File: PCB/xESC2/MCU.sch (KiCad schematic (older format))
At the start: 1 part, among them U4 STM32F405RGTx

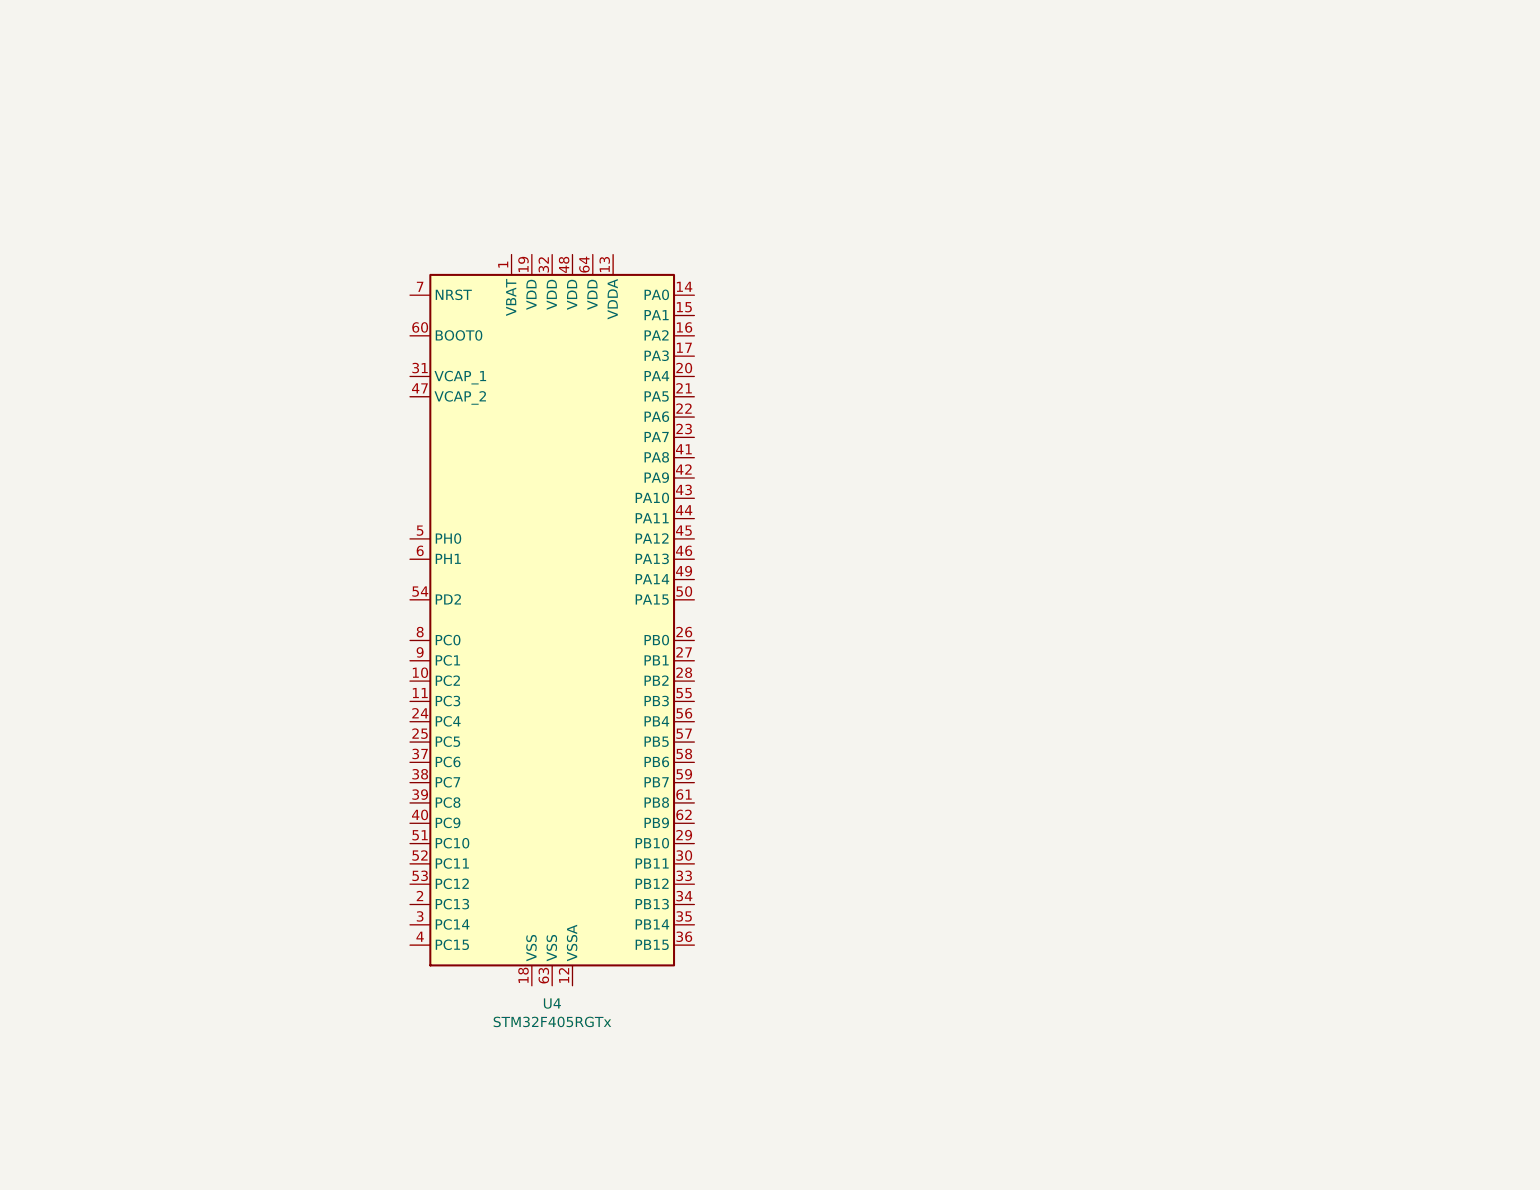
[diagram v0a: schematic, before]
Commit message: wip xESC2 logic
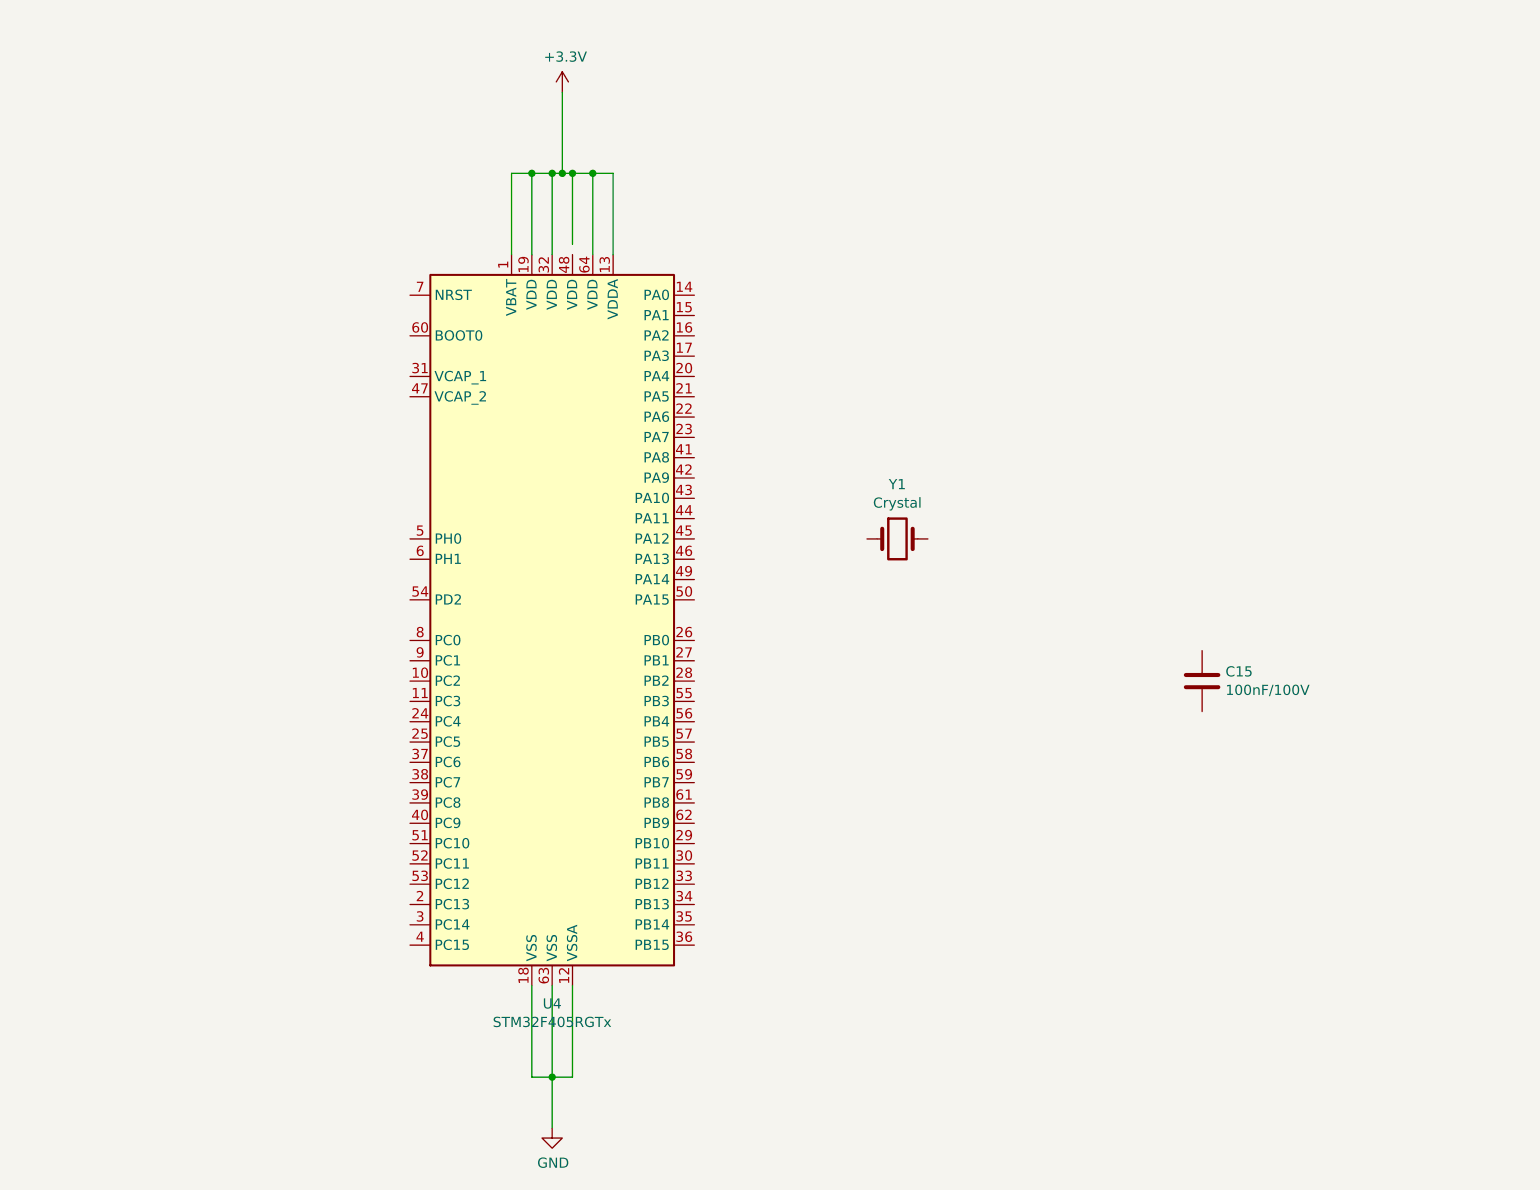
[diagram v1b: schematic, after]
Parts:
- added C15: 100nF/100V, Capacitor_SMD:C_0805_2012Metric, symbol Device:C
- added Y1: Crystal, Crystal:Crystal_SMD_HC49-SD, symbol Device:Crystal
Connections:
- net labels added: +3.3V, GND
- wire segments 0 -> 19
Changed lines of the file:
@@
+	1    0    0    -1
+$EndComp
+Wire Wire Line
+	3250 5150 3250 5600
+Wire Wire Line
+	3250 5600 3350 5600
+Wire Wire Line
+	3450 5600 3450 5150
+Wire Wire Line
+	3350 5150 3350 5600
+Connection ~ 3350 5600
+Wire Wire Line
+	3350 5600 3450 5600
+Wire Wire Line
+	3350 5600 3350 5850
+$Comp
+L power:GND #PWR0123
+U 1 1 61A9A167
+P 3350 5850
+F 0 "#PWR0123" H 3350 5600 50  0001 C CNN
+F 1 "GND" H 3355 5677 50  0000 C CNN
+F 2 "" H 3350 5850 50  0001 C CNN
+F 3 "" H 3350 5850 50  0001 C CNN
+	1    3350 5850
+	1    0    0    -1
+$EndComp
+$Comp
+L Device:C C?
+U 1 1 61A9BC8B
+P 6550 3650
+AR Path="/61A3F4E8/61A9BC8B" Ref="C?"  Part="1"
+AR Path="/61AC26FB/61A9BC8B" Ref="C15"  Part="1"
+F 0 "C15" H 6665 3696 50  0000 L CNN
+F 1 "100nF/100V" H 6665 3605 50  0000 L CNN
+F 2 "Capacitor_SMD:C_0805_2012Metric" H 6588 3500 50  0001 C CNN
+F 3 "~" H 6550 3650 50  0001 C CNN
+	1    6550 3650
+	1    0    0    -1
+$EndComp
+$Comp
+L power:+3.3V #PWR?
+U 1 1 61A9F4B2
+P 3400 750
+AR Path="/61A9F4B2" Ref="#PWR?"  Part="1"
+AR Path="/61AC26FB/61A9F4B2" Ref="#PWR0124"  Part="1"
+F 0 "#PWR0124" H 3400 600 50  0001 C CNN
+F 1 "+3.3V" H 3415 923 50  0000 C CNN
+F 2 "" H 3400 750 50  0001 C CNN
+F 3 "" H 3400 750 50  0001 C CNN
+	1    3400 750
+	1    0    0    -1
+$EndComp
+Wire Wire Line
+	3400 750  3400 1150
+Wire Wire Line
+	3150 1550 3150 1150
+Wire Wire Line
+	3400 1150 3450 1150
+Wire Wire Line
+	3650 1150 3650 1550
+Connection ~ 3400 1150
+Wire Wire Line
+	3550 1550 3550 1150
+Connection ~ 3550 1150
+Wire Wire Line
+	3550 1150 3650 1150
+Wire Wire Line
+	3450 1500 3450 1150
+Connection ~ 3450 1150
+Wire Wire Line
+	3450 1150 3550 1150
+Wire Wire Line
+	3350 1550 3350 1150
+Connection ~ 3350 1150
+Wire Wire Line
+	3350 1150 3400 1150
+Wire Wire Line
+	3250 1550 3250 1150
+Wire Wire Line
+	3150 1150 3250 1150
+Connection ~ 3250 1150
+Wire Wire Line
+	3250 1150 3350 1150
+$Comp
+L Device:Crystal Y1
+U 1 1 61AA35C8
+P 5050 2950
+F 0 "Y1" H 5050 3218 50  0000 C CNN
+F 1 "Crystal" H 5050 3127 50  0000 C CNN
+F 2 "Crystal:Crystal_SMD_HC49-SD" H 5050 2950 50  0001 C CNN
+F 3 "~" H 5050 2950 50  0001 C CNN
+	1    5050 2950
 	1    0    0    -1
 $EndComp

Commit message: wip logic
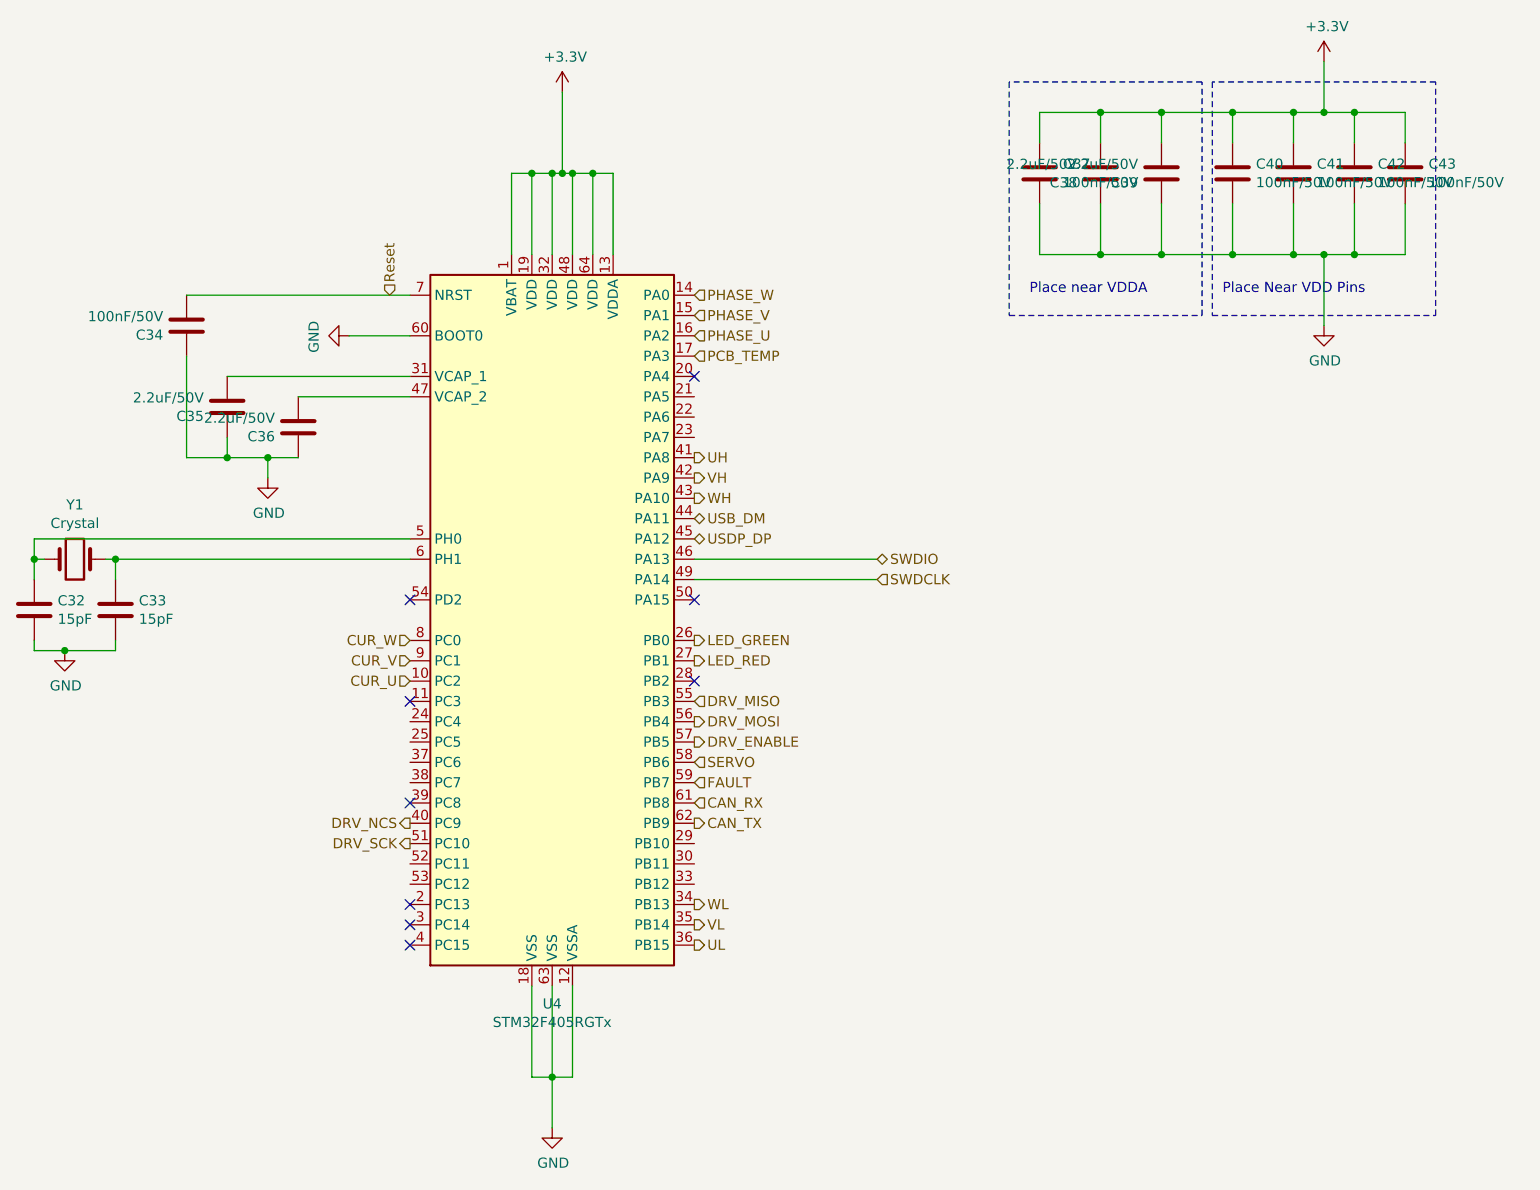
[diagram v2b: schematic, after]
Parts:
- removed C15: 100nF/100V, Capacitor_SMD:C_0805_2012Metric, symbol Device:C
- added C32, C33: 15pF, Capacitor_SMD:C_0603_1608Metric, symbol Device:C
- added C34, C37, C40, C41, C42, C43: 100nF/50V, Capacitor_SMD:C_0603_1608Metric, symbol Device:C
- added C35, C36, C38, C39: 2.2uF/50V, Capacitor_SMD:C_0805_2012Metric, symbol Device:C
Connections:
- net labels added: CAN_RX, CAN_TX, CUR_U, CUR_V, CUR_W, DRV_ENABLE, DRV_MISO, DRV_MOSI, DRV_NCS, DRV_SCK, FAULT, LED_GREEN, LED_RED, PCB_TEMP, PHASE_U, PHASE_V, PHASE_W, Reset, SERVO, SWDCLK, SWDIO, UH, UL, USB_DM, USDP_DP, VH, VL, WH, WL
- wire segments 19 -> 72
- no-connect marks 0 -> 9
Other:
- note added: "Place Near VDD Pins"
- note added: "Place near VDDA"
- moved on the sheet: Y1
